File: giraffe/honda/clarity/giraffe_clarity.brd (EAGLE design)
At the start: 100.3 x 31.8 mm, 6 parts, among them J3 OBDII-FEMALE-CUT, J4 VERT_RJ45, SW1 4XDPSTSMT

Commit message: Fixed ground vias
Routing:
- net GND: vias 1 -> 5
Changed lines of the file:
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@@
 <grid distance="0.025" unitdist="inch" unit="inch" style="dots" multiple="1" display="yes" altdistance="0.0125" altunitdist="inch" altunit="inch"/>
 <layers>
-<layer number="1" name="Top" color="4" fill="1" visible="no" active="yes"/>
+<layer number="1" name="Top" color="4" fill="1" visible="yes" active="yes"/>
 <layer number="2" name="Route2" color="1" fill="3" visible="yes" active="yes"/>
 <layer number="3" name="Route3" color="4" fill="3" visible="no" active="no"/>
@@
 <layer number="14" name="Route14" color="1" fill="6" visible="no" active="no"/>
 <layer number="15" name="Route15" color="4" fill="6" visible="yes" active="yes"/>
-<layer number="16" name="Bottom" color="1" fill="1" visible="no" active="yes"/>
+<layer number="16" name="Bottom" color="1" fill="1" visible="yes" active="yes"/>
 <layer number="17" name="Pads" color="2" fill="1" visible="yes" active="yes"/>
 <layer number="18" name="Vias" color="2" fill="1" visible="yes" active="yes"/>
@@
 <wire x1="75.495" y1="5.325" x2="79.445" y2="5.325" width="0.508" layer="1"/>
 <via x="5.08" y="29.21" extent="1-16" drill="0.35"/>
+<via x="3.175" y="3.175" extent="1-16" drill="0.35"/>
+<via x="16.51" y="13.335" extent="1-16" drill="0.35"/>
+<via x="39.37" y="5.08" extent="1-16" drill="0.35"/>
+<via x="96.52" y="14.605" extent="1-16" drill="0.35"/>
+<wire x1="79.445" y1="5.325" x2="96.52" y2="14.605" width="0" layer="19" extent="1-1"/>
 </signal>
 <signal name="N$3">
@@
 <wire x1="22.956" y1="8.1079625" x2="22.956" y2="22.0498" width="0.254" layer="16"/>
 </signal>
-<signal name="N$1">
-<via x="39.37" y="5.08" extent="1-16" drill="0.35"/>
-</signal>
-<signal name="N$2">
-<via x="96.52" y="14.605" extent="1-16" drill="0.35"/>
-</signal>
-<signal name="N$4">
-<via x="16.51" y="13.335" extent="1-16" drill="0.35"/>
-</signal>
-<signal name="N$5">
-<via x="3.175" y="3.175" extent="1-16" drill="0.35"/>
-</signal>
 </signals>

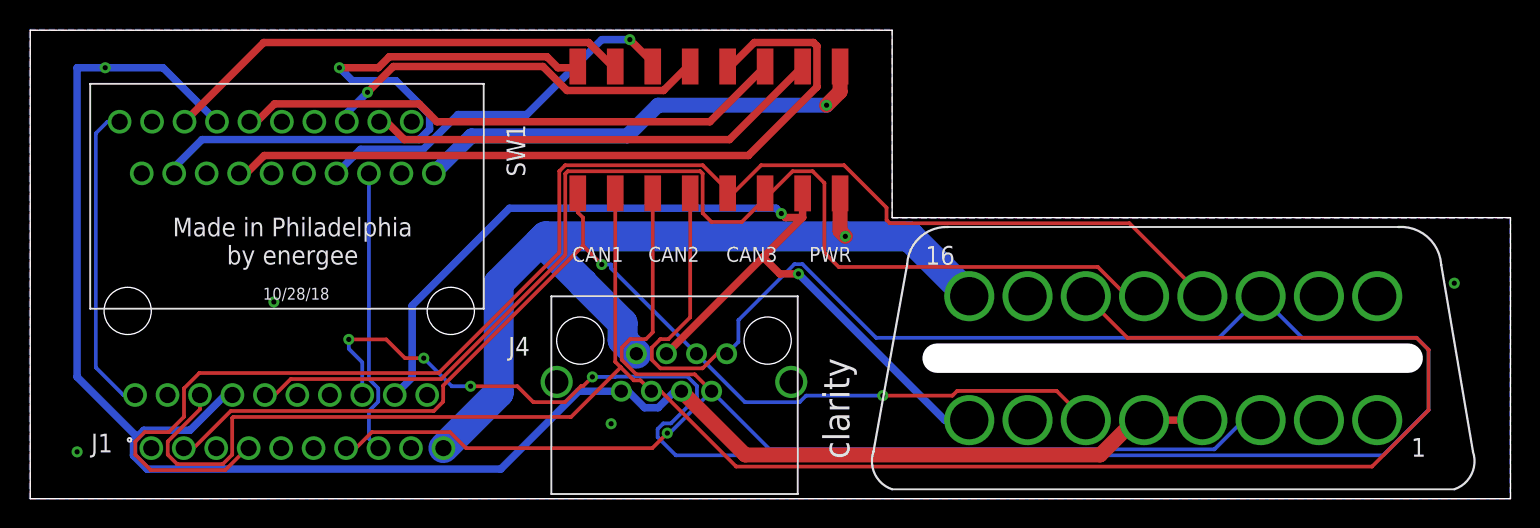
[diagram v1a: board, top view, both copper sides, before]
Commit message: Updated both board traces
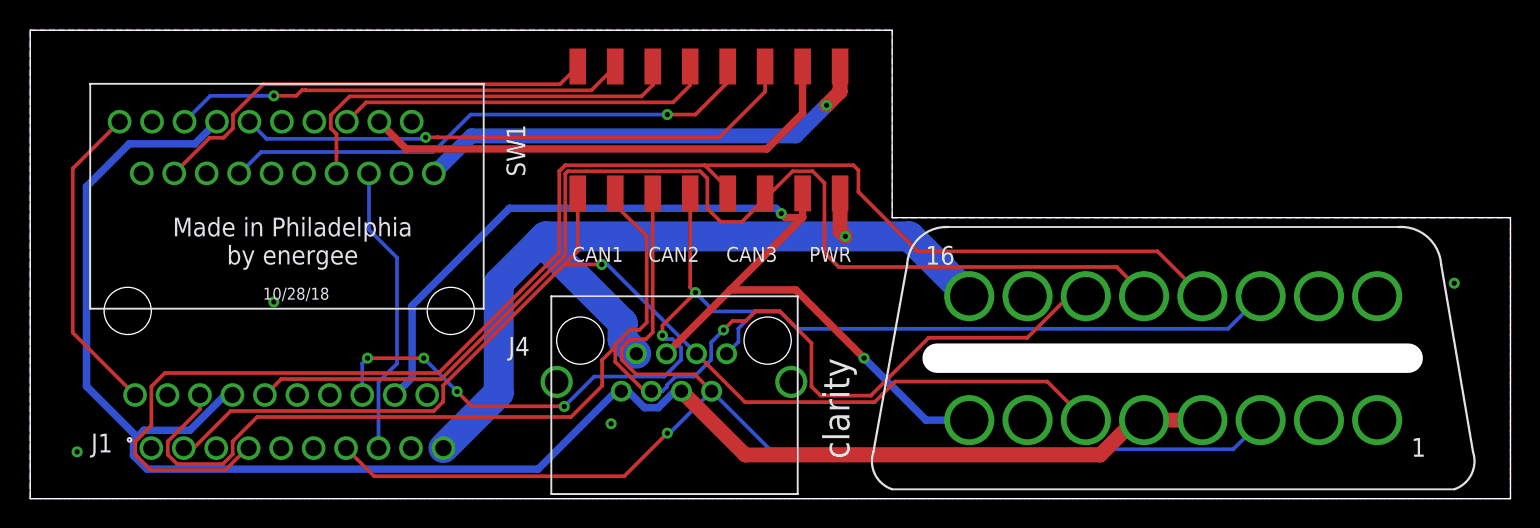
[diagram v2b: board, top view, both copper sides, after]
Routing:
- net CAN2_L: track 167.6 -> 83.6 mm, vias 4 -> 6
- net CAN1_L: track 140.0 -> 96.5 mm, vias 0 -> 1
- net CAN3_H_OUT: track 51.2 -> 36.7 mm, vias 0 -> 1
- net CAN1_H_OUT: track 44.0 -> 30.9 mm, vias 1 -> 0
- net GND: track 125.4 -> 116.8 mm, vias 5 -> 4
- net IGN_OUT: track 31.2 -> 33.6 mm
- net CAN2_H_OUT: track 26.1 -> 28.0 mm, vias 1 -> 0
- net CAN3_H: track 100.0 -> 101.6 mm
- net CAN3_L_OUT: track 37.5 -> 38.9 mm, vias 0 -> 1
- net CAN1_L_OUT: track 32.1 -> 30.8 mm, vias 0 -> 1
- net IGN: track 69.3 -> 70.6 mm
- net CAN2_L_OUT: track 26.5 -> 25.6 mm, vias 1 -> 0
- net CAN1_H: track 76.8 -> 77.7 mm, vias 2 -> 1
- net CAN2_H: track 86.7 -> 87.4 mm
- net LDW_OFF_SW: track 19.4 -> 19.9 mm
